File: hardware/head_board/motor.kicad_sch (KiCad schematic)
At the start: 18 parts, among them J4 MOTOR, U7 TMC2209

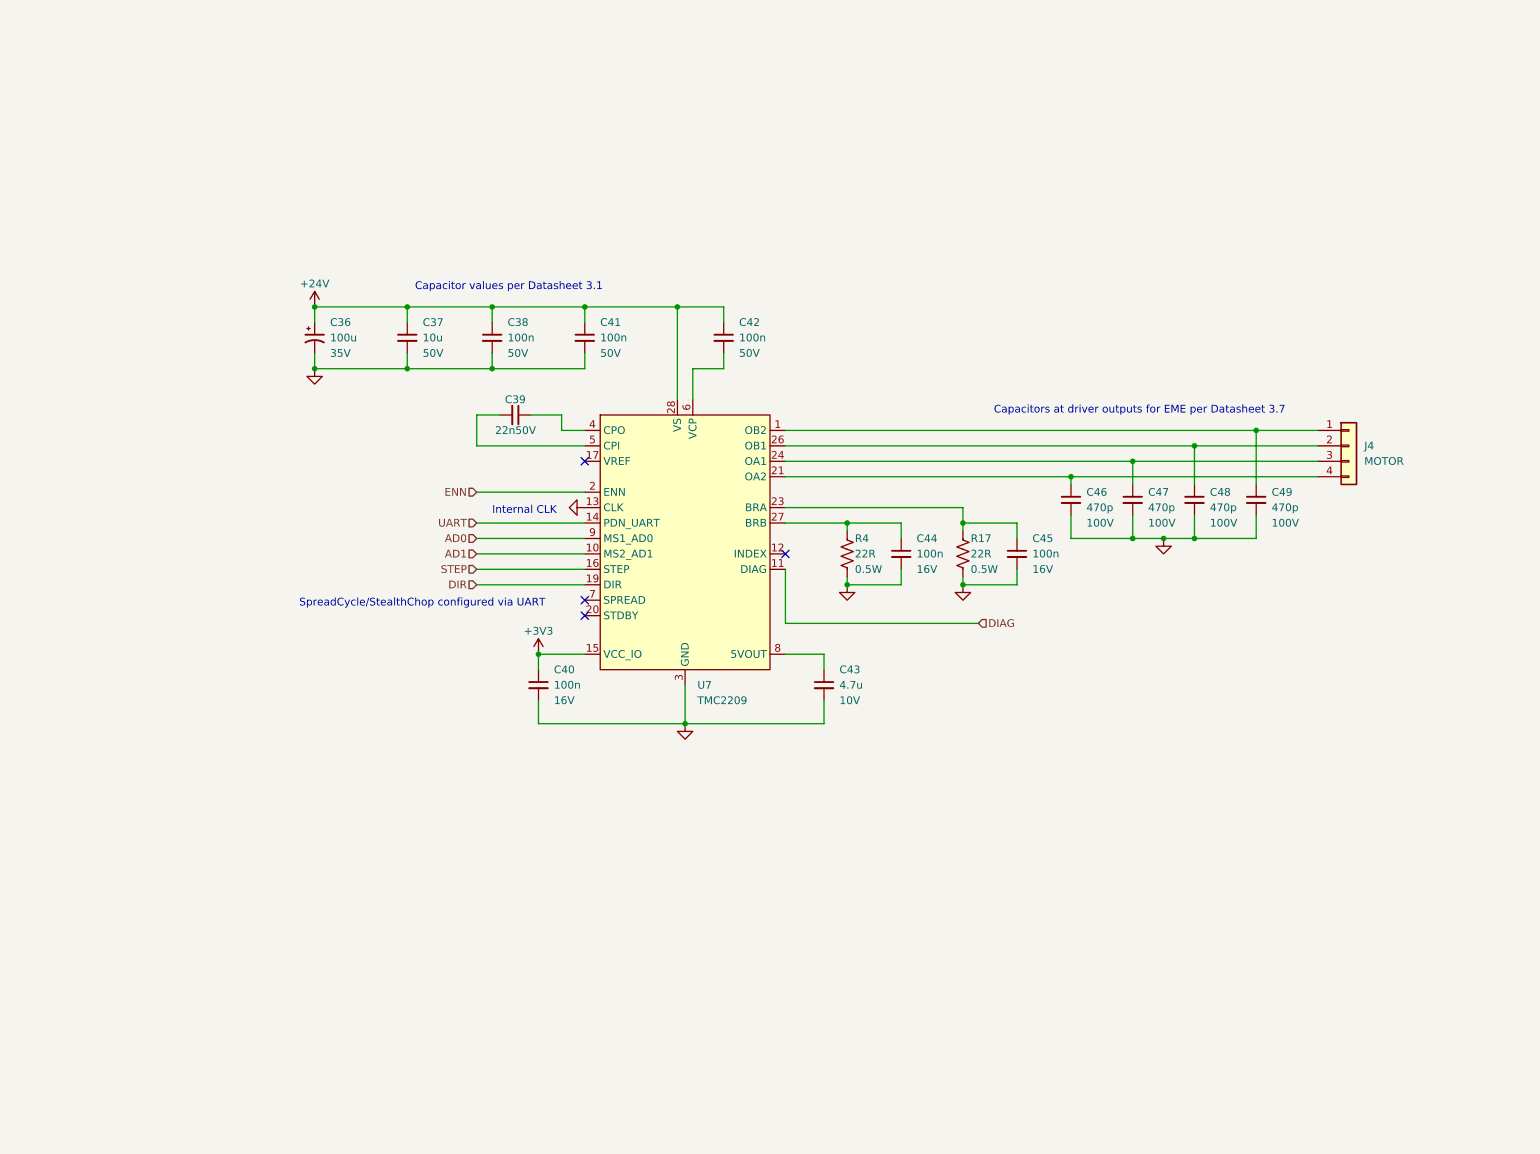
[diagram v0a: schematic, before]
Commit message: v1 revision to the schematic
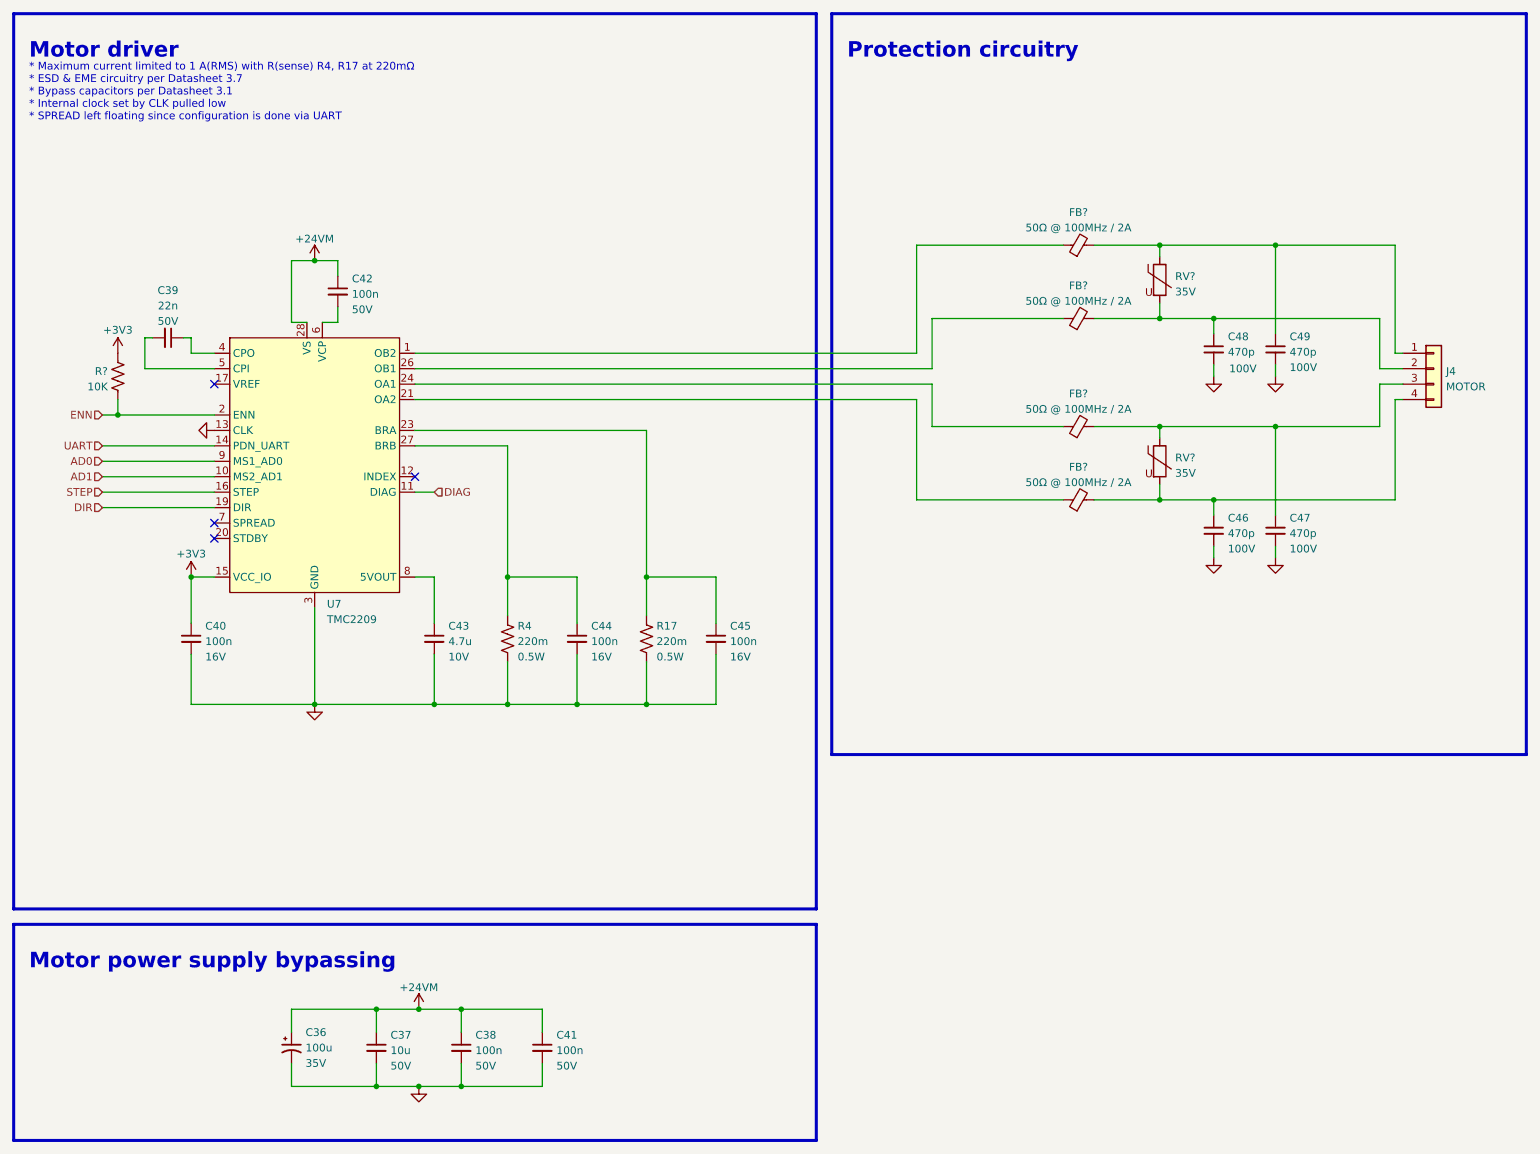
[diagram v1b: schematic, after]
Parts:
- added FB? (x4): 50Ω @ 100MHz / 2A, symbol Device:FerriteBead_Small
- added R?: 10K, Resistor_SMD:R_0402_1005Metric_Pad0.72x0.64mm_HandSolder, symbol Device:R_US
- added RV? (x2): 35V, symbol Device:Varistor
- R17, R4: value 22R -> 220m
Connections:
- net +3V3: now also R?.2
- net ENN: now also R?.1
- net at C48.1, J4.2 (Pin_2): now also FB?.2, RV?.2; no longer U7.26 (OB1)
- net at C46.1, J4.4 (Pin_4): now also FB?.2, RV?.2; no longer U7.21 (OA2)
- net at C49.1, J4.1 (Pin_1): now also FB?.2, RV?.1; no longer U7.1 (OB2)
- net at C47.1, J4.3 (Pin_3): now also FB?.2, RV?.1; no longer U7.24 (OA1)
- new net: FB?.1, U7.26 (OB1)
- new net: FB?.1, U7.1 (OB2)
- new net: FB?.1, U7.21 (OA2)
- new net: FB?.1, U7.24 (OA1)
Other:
- note added: "* Maximum current limited to 1 A(RMS) with R(sense) R4, R17 at 220mΩ * ESD & EME circuitry per Datasheet 3.7 * Bypass capacitors per Datasheet 3.1 * Internal clock set by CLK pulled low * SPREAD left floating since configuration is done via UART"
- note added: "Motor driver"
- note added: "Motor power supply bypassing"
- note added: "Protection circuitry"
- note removed: "Capacitor values per Datasheet 3.1"
- note removed: "Capacitors at driver outputs for EME per Datasheet 3.7"
- note removed: "Internal CLK"
- note removed: "SpreadCycle/StealthChop configured via UART"
- company: (none) -> Winterbloom
- title: (none) -> Candela Head
- moved on the sheet: C36, C37, C38, C39, C40, C41, C42, C43, C44, C45, C46, C47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
